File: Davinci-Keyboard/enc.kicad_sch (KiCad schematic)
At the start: 0 parts

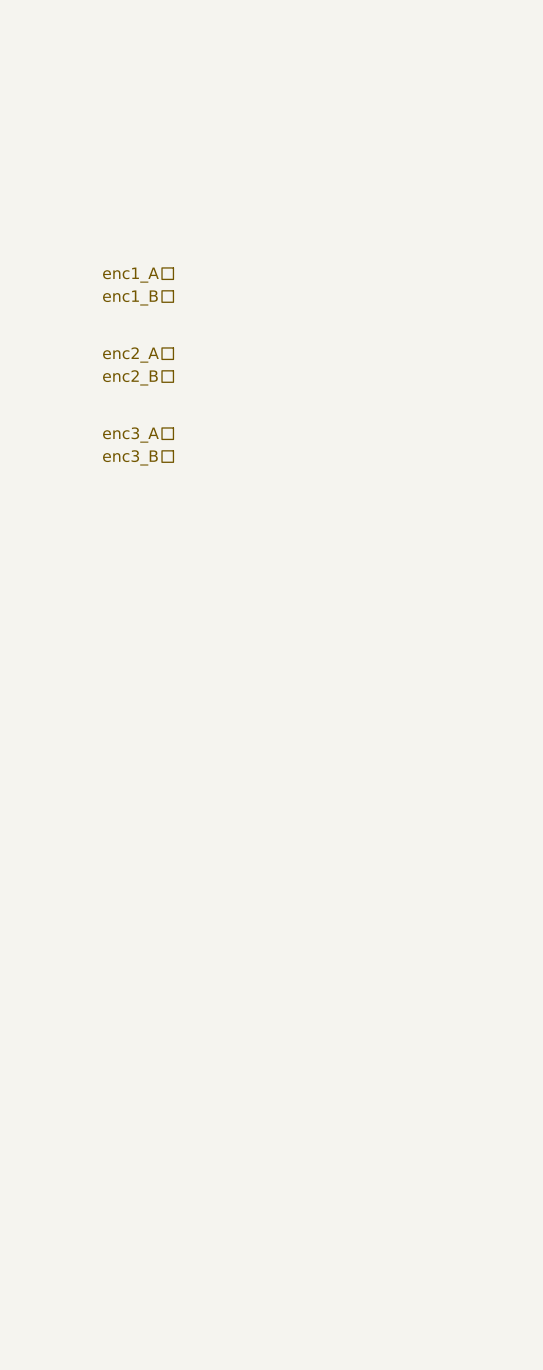
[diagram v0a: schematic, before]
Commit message: 20$越え
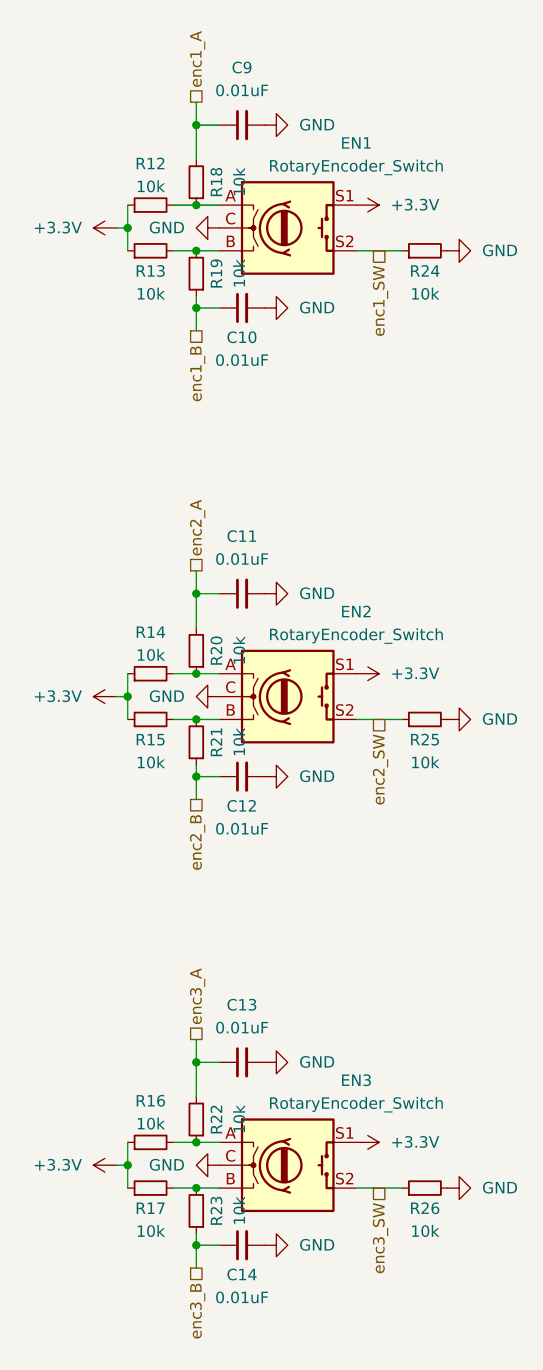
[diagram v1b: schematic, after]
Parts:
- added C10, C11, C12, C13, C14, C9: 0.01uF, Capacitor_SMD:C_0603_1608Metric_Pad1.08x0.95mm_HandSolder, symbol Device:C_Small
- added EN1, EN2, EN3: RotaryEncoder_Switch, BrownSugar_KBD:RotaryEncoder_EC11-Switch, symbol Device:RotaryEncoder_Switch
- added R12, R13, R14, R15, R16, R17, R18, R19, R20, R21, R22, R23, R24, R25, R26: 10k, Resistor_SMD:R_0603_1608Metric_Pad0.98x0.95mm_HandSolder, symbol Device:R_Small
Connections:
- net enc1_A: now also C9.1, R18.2
- net enc1_B: now also C10.1, R19.1
- net enc2_A: now also C11.1, R20.2
- net enc2_B: now also C12.1, R21.1
- net enc3_A: now also C13.1, R22.2
- net enc3_B: now also C14.1, R23.1
- new net: EN1.A, R12.2, R18.1
- new net: EN3.A, R16.2, R22.1
- new net: EN3.B, R17.2, R23.2
- new net: EN2.B, R15.2, R21.2
- new net: EN1.B, R13.2, R19.2
- new net: EN2.A, R14.2, R20.1
- new net +3.3V: EN1.S1, EN2.S1, EN3.S1, R12.1, R13.1, R14.1, R15.1, R16.1, R17.1
- new net GND: C10.2, C11.2, C12.2, C13.2, C14.2, C9.2, EN1.C, EN2.C, EN3.C, R24.2, R25.2, R26.2
- new net enc1_SW: EN1.S2, R24.1
- new net enc2_SW: EN2.S2, R25.1
- new net enc3_SW: EN3.S2, R26.1
